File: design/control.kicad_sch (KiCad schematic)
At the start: 22 parts, among them J1 USB_C_Receptacle_USB2.0_14P, J2 SMB, J3 Conn-OScope, J4 Conn-OScope, J5 SMA, U1 CP2102N-Axx-xQFN20, U2 STM32F303RETx

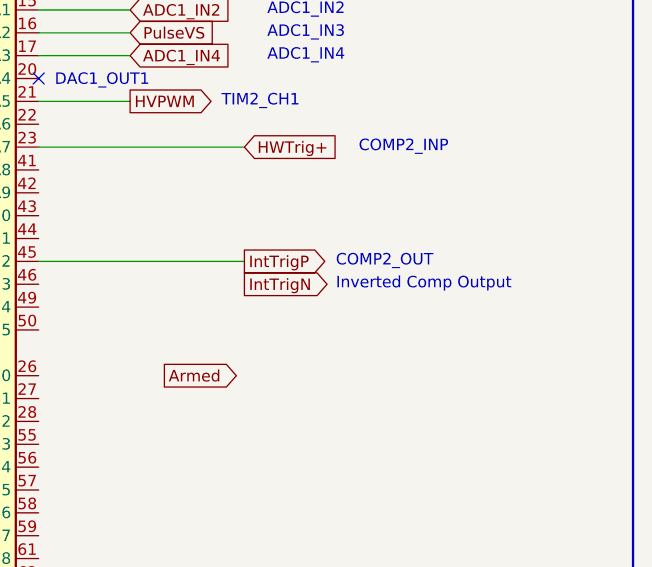
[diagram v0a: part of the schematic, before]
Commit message: _
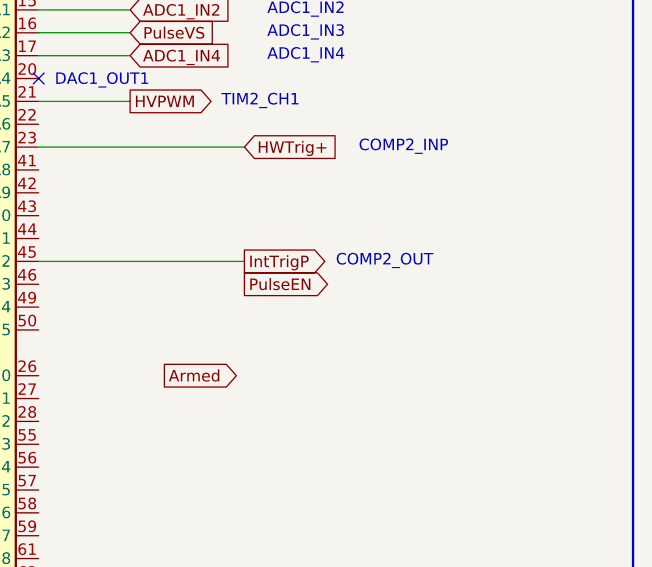
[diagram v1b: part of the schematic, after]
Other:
- note removed: "Inverted Comp Output"
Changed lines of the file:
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@@
-		)
-	)
-	(text "Inverted Comp Output"
-		(exclude_from_sim no)
-		(at 247.65 82.55 0)
-		(effects
-			(font
-				(size 1.27 1.27)
-			)
-			(justify left)
 		)
 	)
@@
 		)
 	)
-	(global_label "IntTrigN"
+	(global_label "PulseEN"
 		(shape output)
 		(at 237.49 82.55 0)
@@
 		)
 		(property "Intersheetrefs" "${INTERSHEET_REFS}"
-			(at 247.7928 82.55 0)
+			(at 248.1556 82.55 0)
 			(effects
 				(font
